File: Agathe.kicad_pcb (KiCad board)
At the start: 2 copper layers, 338.8 x 114.8 mm, 173 parts, among them J1 Conn_01x04_Female, J2 Conn_01x02_Female, J4 Conn_01x02_Female, SW1 SW_Push, U1 ATmega32U4-AU, U2 PRTR5V0U2X, Y1 16MHz

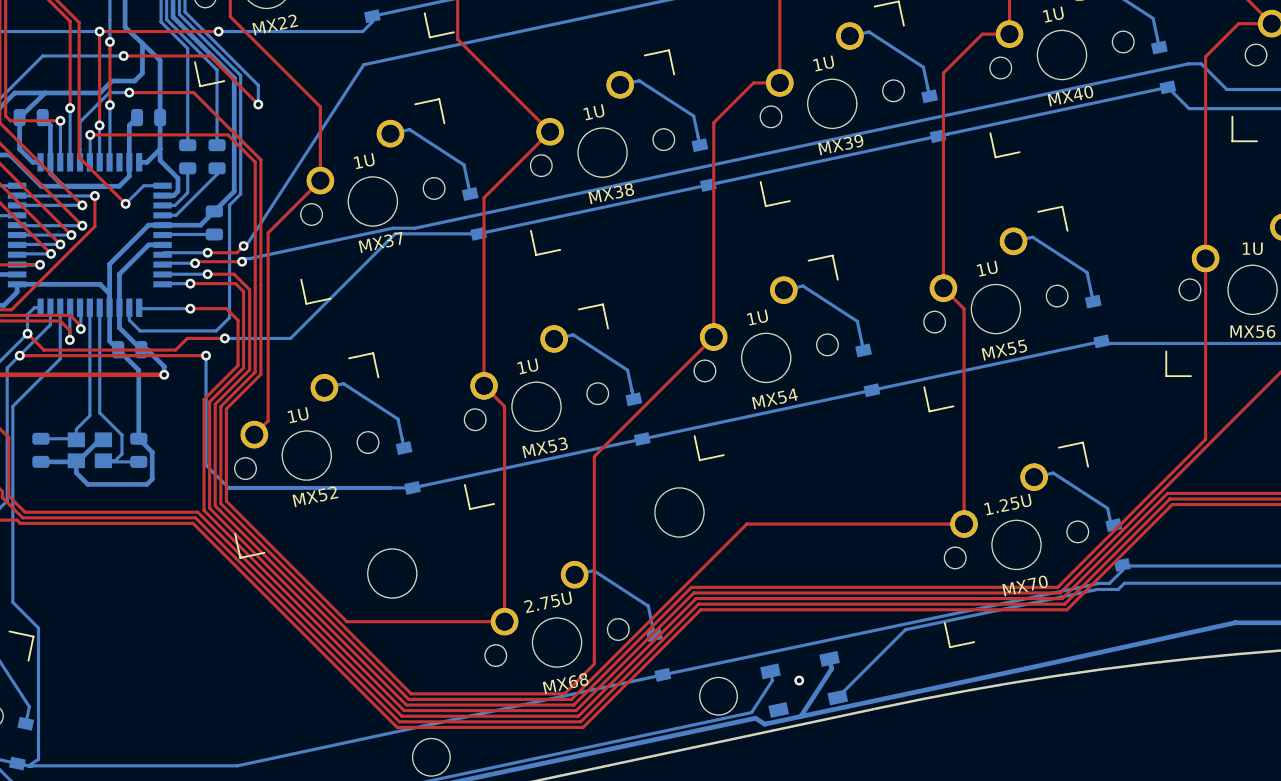
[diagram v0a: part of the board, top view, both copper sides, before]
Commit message: add a capacitor
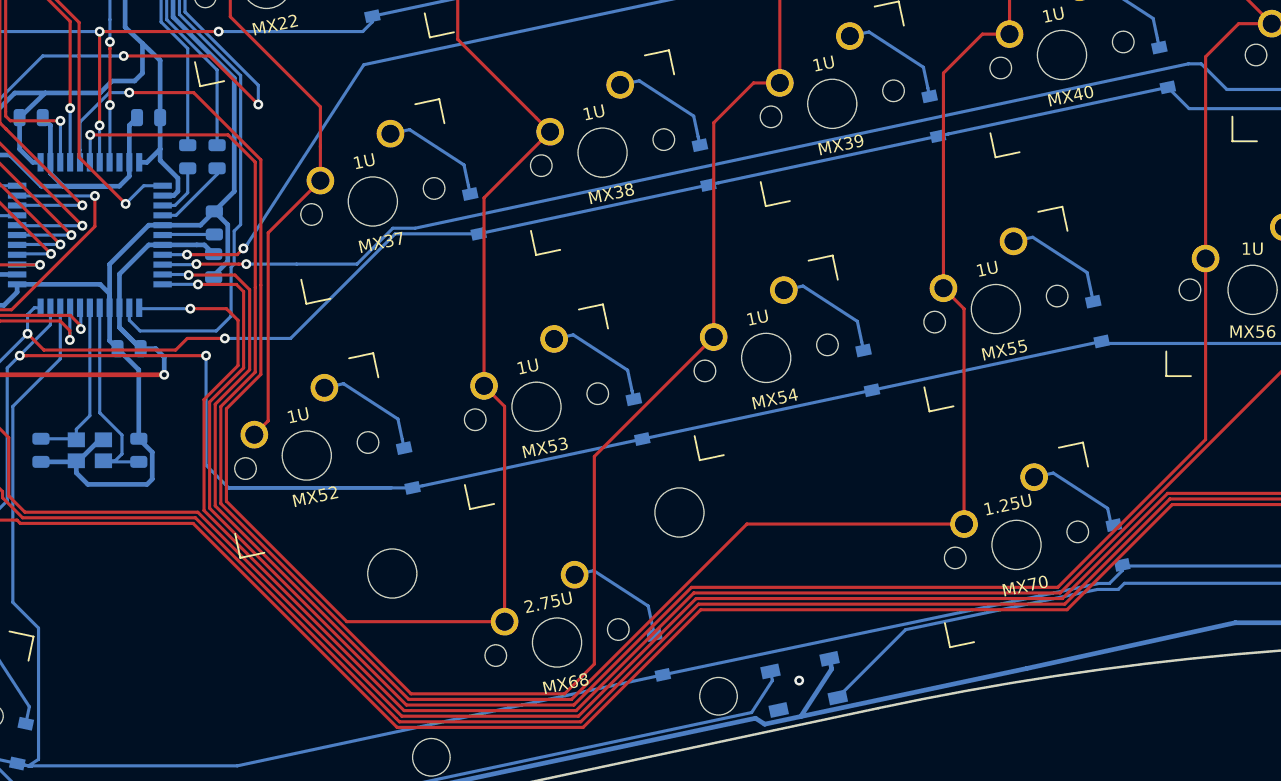
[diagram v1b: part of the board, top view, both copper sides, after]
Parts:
- added C8: 0.1uF, Capacitor_SMD:C_0805_2012Metric, B.Cu at (199.6, 141.7)
- moved C5 9.63 mm to (206.5, 135.0), turned to 270 degrees
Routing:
- net +5V: track 1086.2 -> 1093.4 mm
- net GND: track 264.2 -> 270.3 mm
- net ROTA: track 255.0 -> 255.8 mm
